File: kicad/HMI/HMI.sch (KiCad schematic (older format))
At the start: 38 parts

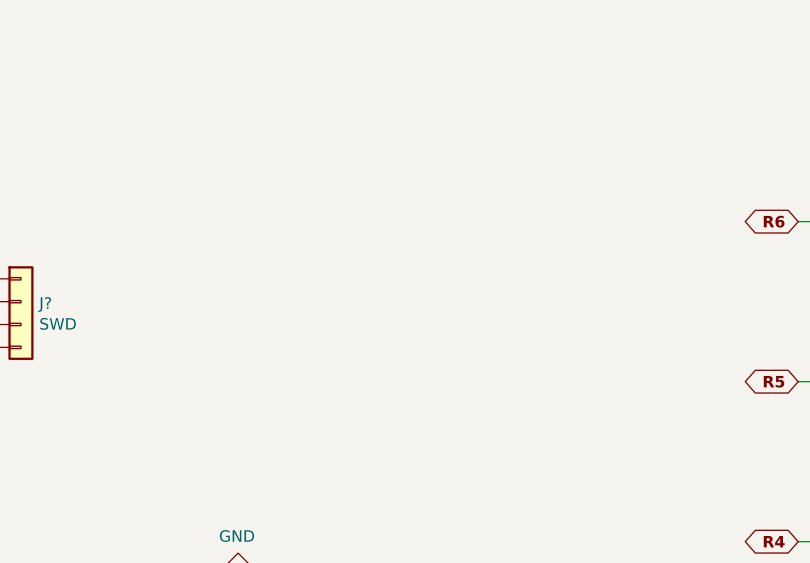
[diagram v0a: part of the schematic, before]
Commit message: Add files via upload
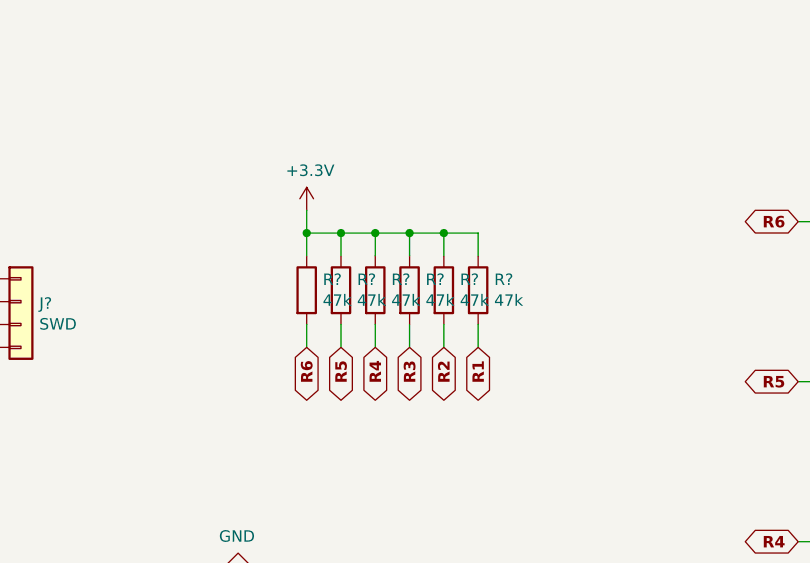
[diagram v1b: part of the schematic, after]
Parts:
- added R? (x6): 47k, symbol Device:R
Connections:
- net +3V3: now also R?.1, R?.1, R?.1, R?.1, R?.1, R?.1
- net R1: now also R?.2
- net R2: now also R?.2
- net R3: now also R?.2
- net R4: now also R?.2
- net R5: now also R?.2
- net R6: now also R?.2
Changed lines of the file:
@@
 	1    0    0    -1
 $EndComp
+Text GLabel 5900 2050 3    50   BiDi ~ 10
+R6
+$Comp
+L Device:R R?
+U 1 1 5E2A8493
+P 5900 1800
+F 0 "R?" H 5970 1846 50  0000 L CNN
+F 1 "47k" H 5970 1755 50  0000 L CNN
+F 2 "" V 5830 1800 50  0001 C CNN
+F 3 "~" H 5900 1800 50  0001 C CNN
+	1    5900 1800
+	1    0    0    -1
+$EndComp
+$Comp
+L power:+3.3V #PWR?
+U 1 1 5E2A8834
+P 5900 1450
+F 0 "#PWR?" H 5900 1300 50  0001 C CNN
+F 1 "+3.3V" H 5915 1623 50  0000 C CNN
+F 2 "" H 5900 1450 50  0001 C CNN
+F 3 "" H 5900 1450 50  0001 C CNN
+	1    5900 1450
+	1    0    0    -1
+$EndComp
+Text GLabel 6050 2050 3    50   BiDi ~ 10
+R5
+Text GLabel 6200 2050 3    50   BiDi ~ 10
+R4
+Text GLabel 6350 2050 3    50   BiDi ~ 10
+R3
+Text GLabel 6500 2050 3    50   BiDi ~ 10
+R2
+Text GLabel 6650 2050 3    50   BiDi ~ 10
+R1
+$Comp
+L Device:R R?
+U 1 1 5E2C0402
+P 6050 1800
+F 0 "R?" H 6120 1846 50  0000 L CNN
+F 1 "47k" H 6120 1755 50  0000 L CNN
+F 2 "" V 5980 1800 50  0001 C CNN
+F 3 "~" H 6050 1800 50  0001 C CNN
+	1    6050 1800
+	1    0    0    -1
+$EndComp
+$Comp
+L Device:R R?
+U 1 1 5E2C057A
+P 6200 1800
+F 0 "R?" H 6270 1846 50  0000 L CNN
+F 1 "47k" H 6270 1755 50  0000 L CNN
+F 2 "" V 6130 1800 50  0001 C CNN
+F 3 "~" H 6200 1800 50  0001 C CNN
+	1    6200 1800
+	1    0    0    -1
+$EndComp
+$Comp
+L Device:R R?
+U 1 1 5E2C0631
+P 6350 1800
+F 0 "R?" H 6420 1846 50  0000 L CNN
+F 1 "47k" H 6420 1755 50  0000 L CNN
+F 2 "" V 6280 1800 50  0001 C CNN
+F 3 "~" H 6350 1800 50  0001 C CNN
+	1    6350 1800
+	1    0    0    -1
+$EndComp
+$Comp
+L Device:R R?
+U 1 1 5E2C075F
+P 6500 1800
+F 0 "R?" H 6570 1846 50  0000 L CNN
+F 1 "47k" H 6570 1755 50  0000 L CNN
+F 2 "" V 6430 1800 50  0001 C CNN
+F 3 "~" H 6500 1800 50  0001 C CNN
+	1    6500 1800
+	1    0    0    -1
+$EndComp
+$Comp
+L Device:R R?
+U 1 1 5E2C0888
+P 6650 1800
+F 0 "R?" H 6720 1846 50  0000 L CNN
+F 1 "47k" H 6720 1755 50  0000 L CNN
+F 2 "" V 6580 1800 50  0001 C CNN
+F 3 "~" H 6650 1800 50  0001 C CNN
+	1    6650 1800
+	1    0    0    -1
+$EndComp
+Wire Wire Line
+	5900 2050 5900 1950
+Wire Wire Line
+	6050 1950 6050 2050
+Wire Wire Line
+	6200 2050 6200 1950
+Wire Wire Line
+	6350 1950 6350 2050
+Wire Wire Line
+	6500 2050 6500 1950
+Wire Wire Line
+	6650 1950 6650 2050
+Wire Wire Line
+	6650 1650 6650 1550
+Wire Wire Line
+	6650 1550 6500 1550
+Wire Wire Line
+	5900 1550 5900 1450
+Wire Wire Line
+	5900 1650 5900 1550
+Connection ~ 5900 1550
+Wire Wire Line
+	6050 1550 6050 1650
+Connection ~ 6050 1550
+Wire Wire Line
+	6050 1550 5900 1550
+Wire Wire Line
+	6200 1550 6200 1650
+Connection ~ 6200 1550
+Wire Wire Line
+	6200 1550 6050 1550
+Wire Wire Line
+	6350 1550 6350 1650
+Connection ~ 6350 1550
+Wire Wire Line
+	6350 1550 6200 1550
+Wire Wire Line
+	6500 1550 6500 1650
+Connection ~ 6500 1550
+Wire Wire Line
+	6500 1550 6350 1550
 $EndSCHEMATC
